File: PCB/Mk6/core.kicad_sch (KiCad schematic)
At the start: 11 parts, among them J3 Bank, J4 Debug, U4 R65C02, U5 EEPROM, U6 62256, U8 GAL20V8B-10

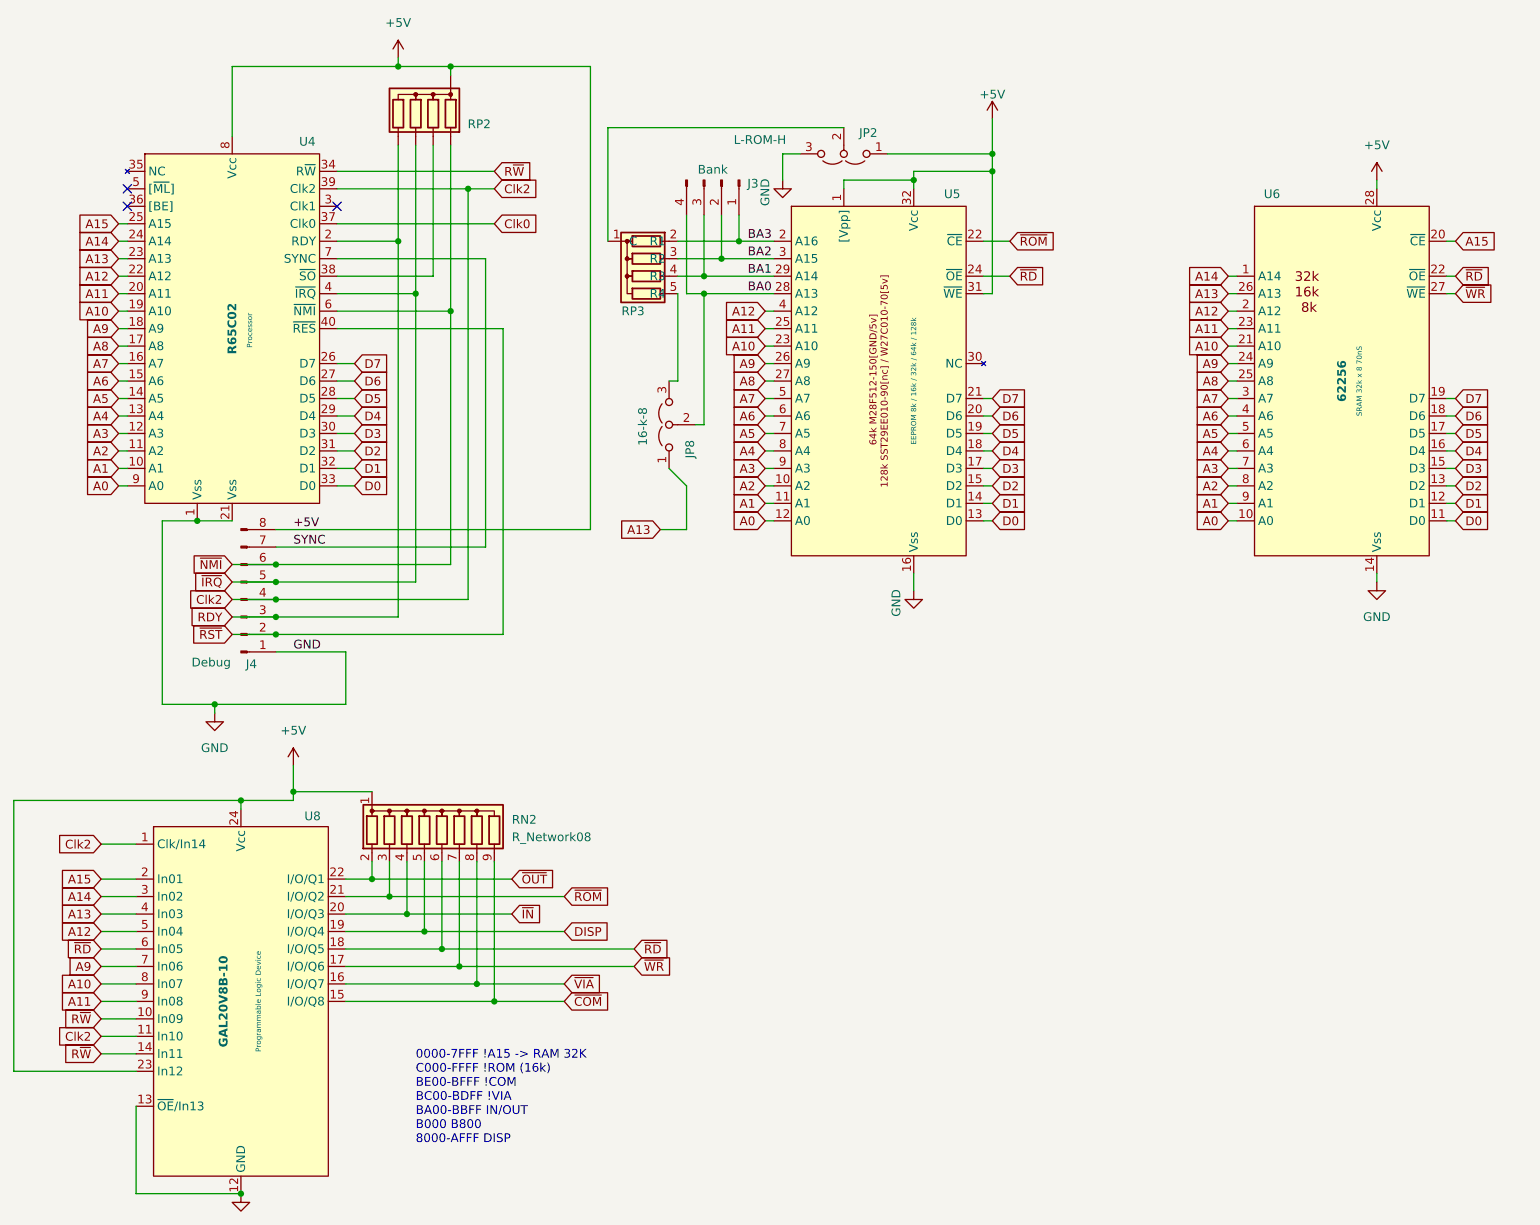
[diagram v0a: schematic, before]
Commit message: Pre Remap
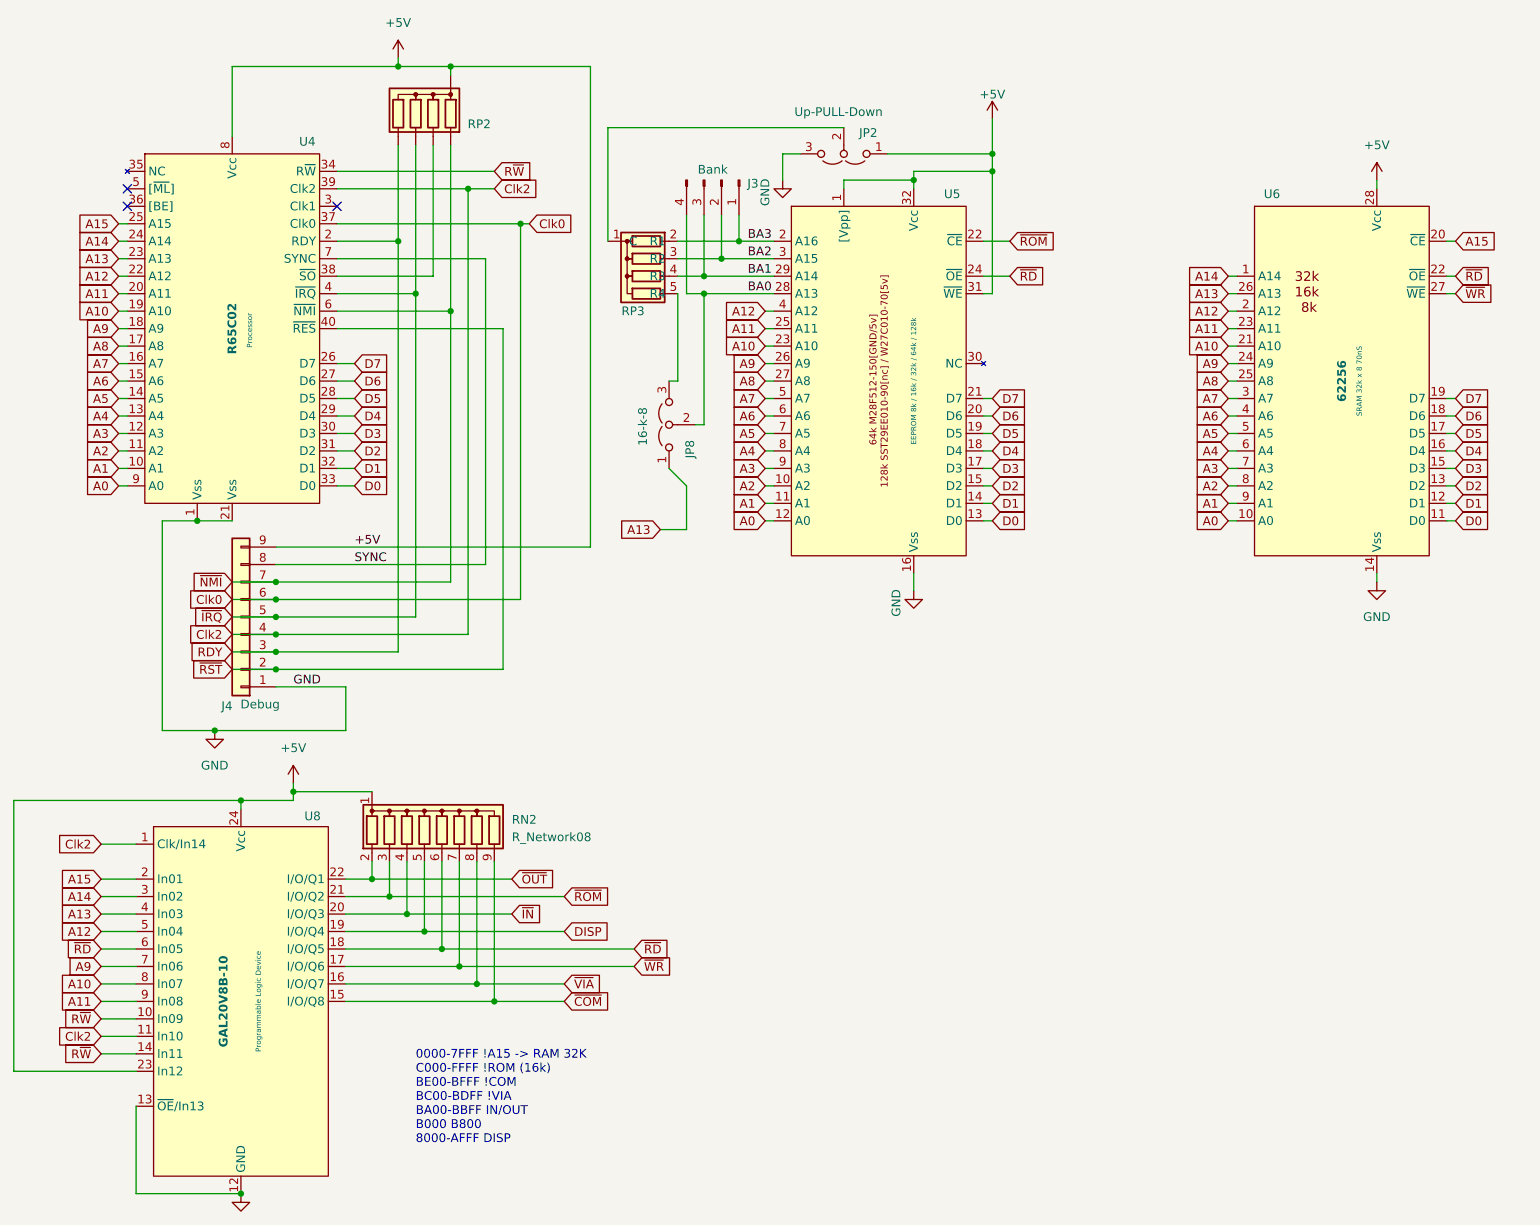
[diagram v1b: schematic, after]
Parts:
- removed J4: Debug, Connector_PinHeader_2.54mm:PinHeader_1x08_P2.54mm_Vertical, symbol Connector:Conn_01x08_Pin
- added J4: Debug, Connector_PinHeader_2.54mm:PinHeader_1x09_P2.54mm_Vertical, symbol Connector_Generic:Conn_01x09
- JP2: value L-ROM-H -> Up-PULL-Down
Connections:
- net +5V: now also J4.9 (Pin_9)
- net Clk0: now also J4.6 (Pin_6)
- net Clk2: now also J4.4 (Pin_4)
- net GND: now also J4.1 (Pin_1)
- net RDY: now also J4.3 (Pin_3)
- net SYNC: now also J4.8 (Pin_8)
- net ~{IRQ}: now also J4.5 (Pin_5)
- net ~{NMI}: now also J4.7 (Pin_7)
- net ~{RST}: now also J4.2 (Pin_2)
